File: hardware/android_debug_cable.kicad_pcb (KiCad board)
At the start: 2 copper layers, 36.7 x 12.2 mm, 11 parts, among them P1 USB_A, P2 CONN_01X04, P3 SJ-43514-SMT-TR, U1 TPS71718DCKR, U2 CP2103-GM

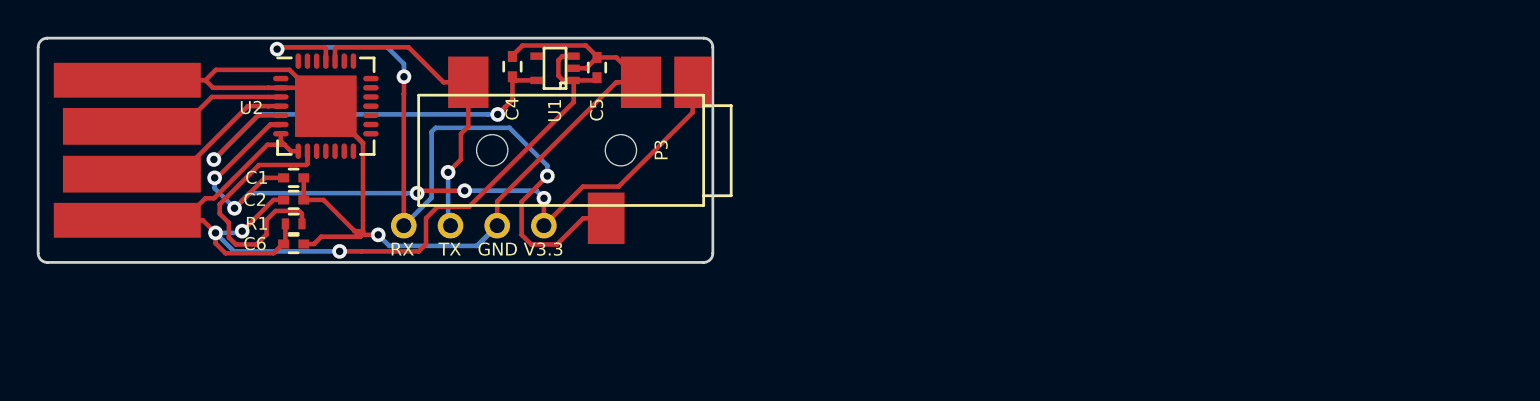
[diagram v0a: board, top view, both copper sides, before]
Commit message: Add first version of v0.4
Signed-off-by: Robert Foss <robert.foss@collabora.com>
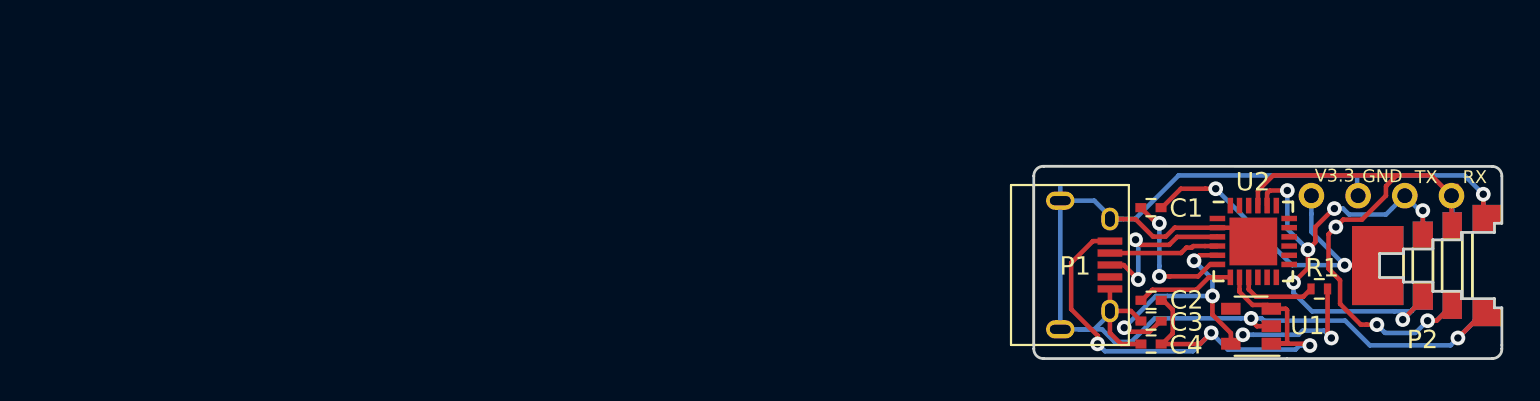
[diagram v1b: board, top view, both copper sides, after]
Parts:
- removed C5: 1uF, Capacitors_SMD:C_0402
- removed C6: 0.1uF, Capacitors_SMD:C_0402
- added C3: 1uF, Capacitors_SMD:C_0402, F.Cu at (138.8, 91.7)
- added G***: LOGO, memcpy_logo:memcpy_logo_13.2x3.6mm, B.Cu at (139.6, 88.8)
- C1: value 0.1uF -> 1uF
- P1: value USB_A -> USB_OTG; footprint connectors:usb-PCB -> Connectors:USB_Micro-B
- P2: value CONN_01X04 -> 50-00397; footprint footprints:CONN_2.54mm_1x4_no-outline -> 50-00397:50-00397
- P3: value SJ-43514-SMT-TR -> CONN_01X04; footprint 3-5mm_4pole_jack:3.5mm_4pin_jack -> footprints:CONN_2.54mm_1x4_no-outline
- R1: value 10k -> 1k
- U1: value TPS71718DCKR -> TCR2EF18; footprint TO_SOT_Packages_SMD:SC-70-5 -> TO_SOT_Packages_SMD:SOT-23-5
- U2: value CP2103-GM -> CP2102N-A01-GQFN24; footprint Housings_DFN_QFN:QFN-28-1EP_5x5mm_Pitch0.5mm -> Housings_DFN_QFN:QFN-24-1EP_4x4mm_Pitch0.5mm
- moved P1 57.3 mm to (135.2, 88.6)
- moved P2 55.9 mm to (157.9, 86.5), turned to 0 degrees
- moved R1 55.9 mm to (148.0, 89.9)
- moved U2 51.0 mm to (144.4, 87.4)
- moved C2 47.0 mm to (138.8, 90.6), turned to 0 degrees
- moved C1 46.7 mm to (138.8, 85.5), turned to 0 degrees
- moved U1 40.4 mm to (144.3, 92.0), turned to 180 degrees
- moved C4 37.9 mm to (138.8, 92.9), turned to 180 degrees
- moved P3 37.2 mm to (151.4, 84.9), turned to 0 degrees
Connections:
- C1 pad 1: GND -> Net-(C1-Pad1)
- C2 pad 1: GND -> Net-(C2-Pad1)
- C4 pad 1: V1.8 -> VCC
- P1 pad 4: GND -> (no net)
- P2 pad 1: RX -> V3.3
- P2 pad 3: GND -> RX
- P2 pad 4: V3.3 -> GND
- P3 pad 1: V3.3 -> RX
- P3 pad 3: RX -> GND
- P3 pad 4: GND -> V3.3
- R1 pad 1: VCC -> Net-(R1-Pad1)
- R1 pad 2: Net-(R1-Pad2) -> V1.8
- U2 pad 20: (no net) -> TX
- U2 pad 21: (no net) -> RX
- U2 pad 24: TX -> (no net)
- U2 pad 25: RX -> GND
- U2 pad 6: V3.3 -> Net-(C1-Pad1)
- U2 pad 7: VCC -> Net-(C2-Pad1)
- U2 pad 9: Net-(R1-Pad2) -> Net-(R1-Pad1)
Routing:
- net VCC: track 56.6 -> 35.1 mm
- net V3.3: track 42.0 -> 23.9 mm, vias 5 -> 2
- net GND: track 73.9 -> 88.7 mm, vias 1 -> 3
- net Net-(R1-Pad2): track 14.8 -> 0.00 mm
- net TX: track 17.1 -> 31.1 mm, vias 1 -> 6
- net Net-(C1-Pad1): track 0.00 -> 7.94 mm, vias 0 -> 2
- net RX: track 42.2 -> 36.1 mm
- net Net-(C2-Pad1): track 0.00 -> 5.38 mm
- net Net-(R1-Pad1): track 0.00 -> 4.39 mm
- net USB_D-: track 9.63 -> 6.01 mm
- net V1.8: track 25.3 -> 23.6 mm, vias 2 -> 5
- net USB_D+: track 8.76 -> 9.10 mm, vias 0 -> 2
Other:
- board size 36.7 x 12.2 mm -> 25.5 x 10.5 mm
- board text added: "v0.4"
- board text removed: "1.8V"
- board text removed: "Android Debug Cable v0.2"
- board text removed: "USB to UART VCC 3.3V VIO"
